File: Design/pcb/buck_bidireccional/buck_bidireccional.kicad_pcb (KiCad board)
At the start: 2 copper layers, 85 x 60 mm, 19 parts, among them J1 Conn_01x02_Pin, J2 Screw_Terminal_01x02, J3 Screw_Terminal_01x02, J4 Conn_01x02_Pin, Q1 NMOS, Q2 NMOS, U1 IR2184

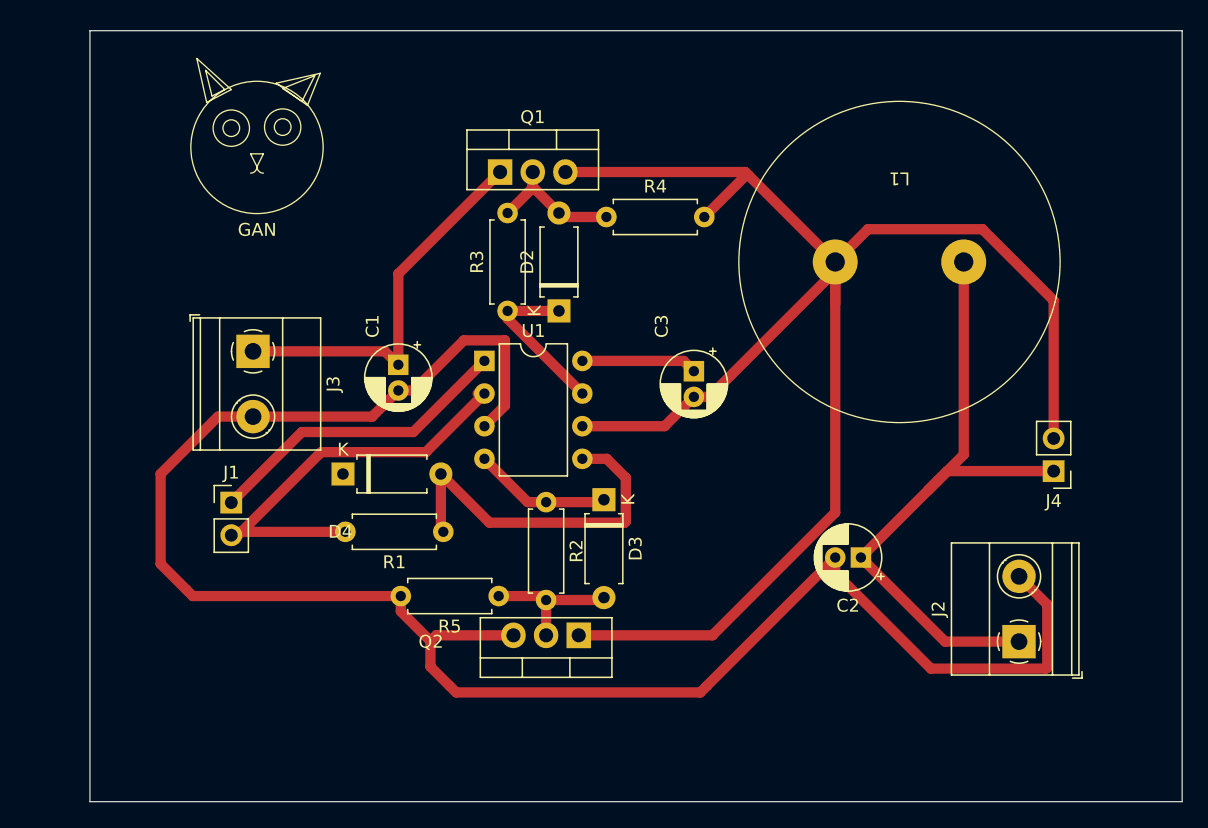
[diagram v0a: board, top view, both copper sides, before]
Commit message: updated pcb
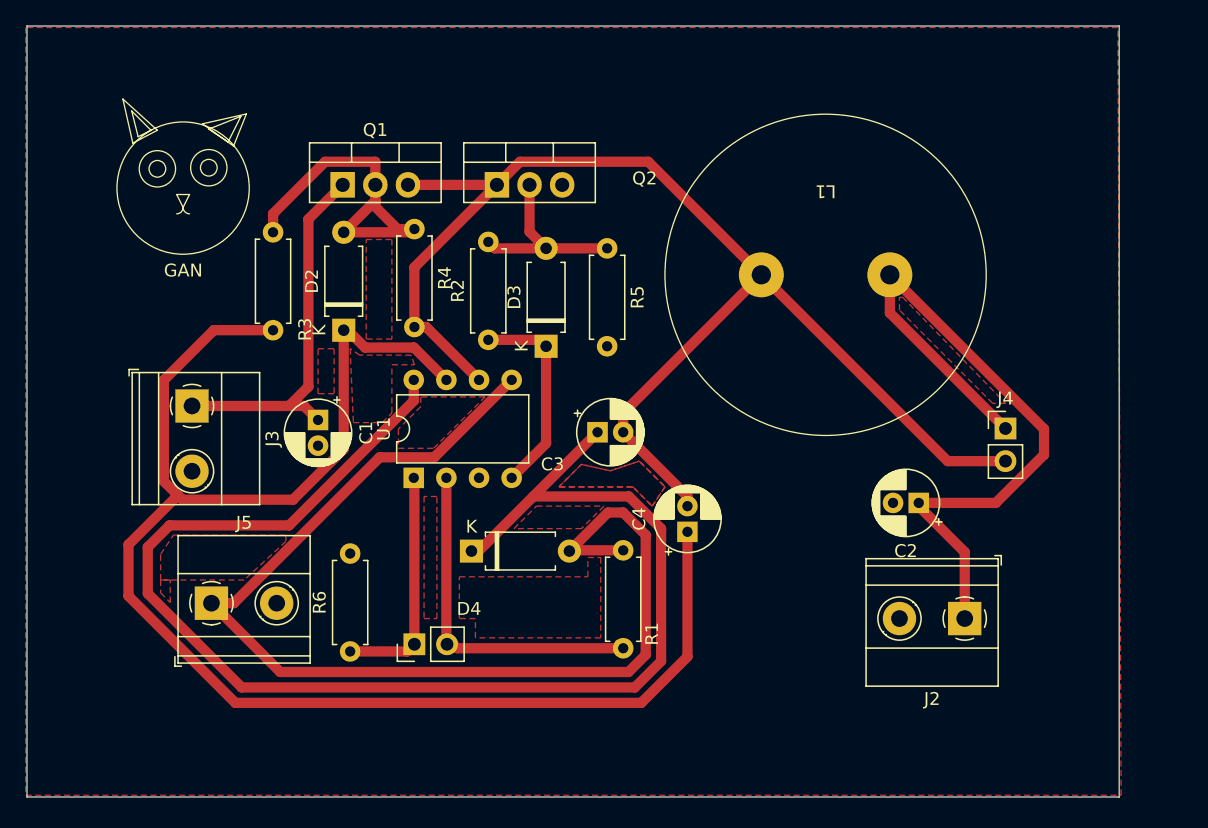
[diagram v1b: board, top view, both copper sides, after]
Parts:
- added C4: 4.7u, Capacitor_THT:CP_Radial_D5.0mm_P2.00mm, F.Cu at (154.5, 120.5)
- added J5: Screw_Terminal_01x02, TerminalBlock_Phoenix:TerminalBlock_Phoenix_MKDS-1,5-2-5.08_1x02_P5.08mm_Horizontal, F.Cu at (117.5, 126.1)
- added R6: 10k, Resistor_THT:R_Axial_DIN0207_L6.3mm_D2.5mm_P7.62mm_Horizontal, F.Cu at (128.2, 129.8)
- R4, R5: value 100k -> 10k
- moved Q2 35.6 mm to (139.7, 93.5), turned to 0 degrees
- moved R5 28.3 mm to (148.2, 98.4), turned to -90 degrees
- moved R3 18.3 mm to (122.2, 104.8)
- moved J1 18.0 mm to (133.2, 129.2), turned to 90 degrees
- moved D2 16.8 mm to (127.8, 104.8)
- moved R4 15.0 mm to (133.2, 96.9), turned to -90 degrees
- moved R1 14.1 mm to (149.5, 121.9), turned to -90 degrees
- moved R2 13.4 mm to (139.0, 105.6), turned to 90 degrees
- moved D3 12.8 mm to (143.5, 106.1), turned to 90 degrees
- moved Q1 12.3 mm to (127.7, 93.5)
- moved D4 11.7 mm to (137.7, 122.0)
- moved U1 10.6 mm to (133.2, 116.3), turned to 90 degrees
- moved C3 8.88 mm to (147.5, 112.8), turned to 0 degrees
- moved C1 7.58 mm to (125.8, 111.8)
- moved J3 6.37 mm to (115.9, 110.7)
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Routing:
- net GND: track 143.8 -> 0.00 mm
- net Net-(D2-K): track 12.8 -> 120.6 mm
- net Net-(D4-K): track 9.27 -> 109.4 mm
- net +12V: track 28.0 -> 88.6 mm
- net Net-(J4-Pin_2): track 132.8 -> 101.9 mm
- net Net-(D2-A): track 11.9 -> 27.4 mm
- net Net-(J1-Pin_2): track 33.8 -> 27.6 mm
- net Net-(J1-Pin_1): track 24.3 -> 18.6 mm
- net Net-(D3-K): track 10.8 -> 16.1 mm
- net Net-(J2-Pin_1): track 51.7 -> 56.4 mm
- net Net-(D3-A): track 11.1 -> 14.9 mm
- net Net-(J3-Pin_1): track 30.0 -> 29.2 mm
- added copper zone on F.Cu, net (none)
- added copper zone on F.Cu, net GND
